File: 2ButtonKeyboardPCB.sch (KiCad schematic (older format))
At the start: 14 parts

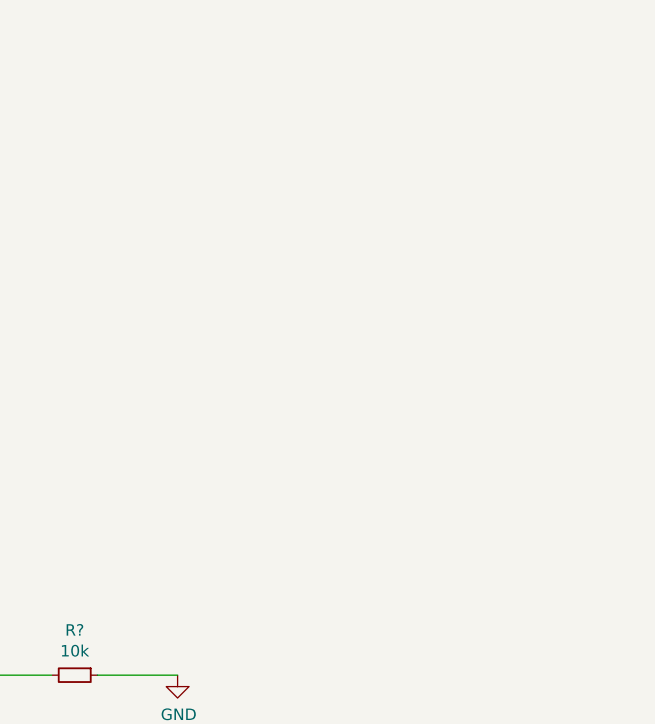
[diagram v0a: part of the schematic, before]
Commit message: Schematic
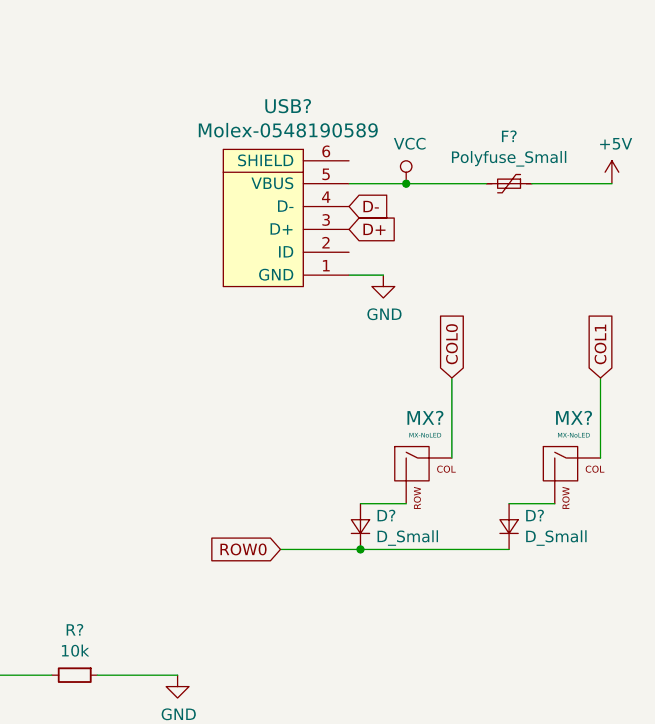
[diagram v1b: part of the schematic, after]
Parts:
- added D? (x2): D_Small, symbol Device:D_Small
- added F?: Polyfuse_Small, symbol Device:Polyfuse_Small
- added MX? (x2): MX-NoLED, symbol MX_Alps_Hybrid:MX-NoLED
- added USB?: Molex-0548190589, symbol random-keyboard-parts:Molex-0548190589
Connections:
- net +5V: now also F?.1
- net D+: now also USB?.3 (D+)
- net D-: now also USB?.4 (D-)
- net GND: now also USB?.1 (GND)
- new net: D?.2 (A), MX?.2 (ROW) (x2)
- new net COL0: MX?.1 (COL)
- new net COL1: MX?.1 (COL)
- new net ROW0: D?.1 (K), D?.1 (K)
- new net VCC: F?.2, USB?.5 (VBUS)
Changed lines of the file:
@@
 Text GLabel 4250 3150 0    50   Input ~ 0
 D-
+$Comp
+L random-keyboard-parts:Molex-0548190589 USB?
+U 1 1 63CE0F7D
+P 8100 2200
+F 0 "USB?" V 8637 2167 60  0000 C CNN
+F 1 "Molex-0548190589" V 8531 2167 60  0000 C CNN
+F 2 "" H 8100 2200 60  0001 C CNN
+F 3 "" H 8100 2200 60  0001 C CNN
+	1    8100 2200
+	0    -1   -1   0
+$EndComp
+$Comp
+L power:VCC #PWR?
+U 1 1 63CE60A6
+P 8650 2000
+F 0 "#PWR?" H 8650 1850 50  0001 C CNN
+F 1 "VCC" H 8667 2173 50  0000 C CNN
+F 2 "" H 8650 2000 50  0001 C CNN
+F 3 "" H 8650 2000 50  0001 C CNN
+	1    8650 2000
+	1    0    0    -1
+$EndComp
+Wire Wire Line
+	8400 2000 8650 2000
+$Comp
+L Device:Polyfuse_Small F?
+U 1 1 63CE9399
+P 9100 2000
+F 0 "F?" V 8895 2000 50  0000 C CNN
+F 1 "Polyfuse_Small" V 8986 2000 50  0000 C CNN
+F 2 "" H 9150 1800 50  0001 L CNN
+F 3 "~" H 9100 2000 50  0001 C CNN
+	1    9100 2000
+	0    1    1    0
+$EndComp
+Wire Wire Line
+	8650 2000 9000 2000
+Connection ~ 8650 2000
+$Comp
+L power:+5V #PWR?
+U 1 1 63CEB500
+P 9550 2000
+F 0 "#PWR?" H 9550 1850 50  0001 C CNN
+F 1 "+5V" H 9565 2173 50  0000 C CNN
+F 2 "" H 9550 2000 50  0001 C CNN
+F 3 "" H 9550 2000 50  0001 C CNN
+	1    9550 2000
+	1    0    0    -1
+$EndComp
+Wire Wire Line
+	9200 2000 9550 2000
+Text GLabel 8400 2200 2    50   Input ~ 0
+D+
+Text GLabel 8400 2100 2    50   Input ~ 0
+D-
+$Comp
+L power:GND #PWR?
+U 1 1 63CED46D
+P 8550 2400
+F 0 "#PWR?" H 8550 2150 50  0001 C CNN
+F 1 "GND" H 8555 2227 50  0000 C CNN
+F 2 "" H 8550 2400 50  0001 C CNN
+F 3 "" H 8550 2400 50  0001 C CNN
+	1    8550 2400
+	1    0    0    -1
+$EndComp
+Wire Wire Line
+	8400 2400 8550 2400
+$Comp
+L MX_Alps_Hybrid:MX-NoLED MX?
+U 1 1 63CEF074
+P 8700 3250
+F 0 "MX?" H 8733 3473 60  0000 C CNN
+F 1 "MX-NoLED" H 8733 3399 20  0000 C CNN
+F 2 "" H 8075 3225 60  0001 C CNN
+F 3 "" H 8075 3225 60  0001 C CNN
+	1    8700 3250
+	1    0    0    -1
+$EndComp
+$Comp
+L Device:D_Small D?
+U 1 1 63CF120D
+P 8450 3500
+F 0 "D?" V 8496 3432 50  0000 R CNN
+F 1 "D_Small" V 8405 3432 50  0000 R CNN
+F 2 "" V 8450 3500 50  0001 C CNN
+F 3 "~" V 8450 3500 50  0001 C CNN
+	1    8450 3500
+	0    -1   -1   0
+$EndComp
+Wire Wire Line
+	8650 3400 8450 3400
+$Comp
+L MX_Alps_Hybrid:MX-NoLED MX?
+U 1 1 63CF6D29
+P 9350 3250
+F 0 "MX?" H 9383 3473 60  0000 C CNN
+F 1 "MX-NoLED" H 9383 3399 20  0000 C CNN
+F 2 "" H 8725 3225 60  0001 C CNN
+F 3 "" H 8725 3225 60  0001 C CNN
+	1    9350 3250
+	1    0    0    -1
+$EndComp
+$Comp
+L Device:D_Small D?
+U 1 1 63CF6D33
+P 9100 3500
+F 0 "D?" V 9146 3432 50  0000 R CNN
+F 1 "D_Small" V 9055 3432 50  0000 R CNN
+F 2 "" V 9100 3500 50  0001 C CNN
+F 3 "~" V 9100 3500 50  0001 C CNN
+	1    9100 3500
+	0    -1   -1   0
+$EndComp
+Wire Wire Line
+	9300 3400 9100 3400
+Wire Wire Line
+	9100 3600 8450 3600
+Connection ~ 8450 3600
+Wire Wire Line
+	8450 3600 8100 3600
+Wire Wire Line
+	8850 3200 8850 2850
+Wire Wire Line
+	9500 3200 9500 2850
+Text GLabel 8850 2850 1    50   Input ~ 0
+COL0
+Text GLabel 9500 2850 1    50   Input ~ 0
+COL1
+Text GLabel 8100 3600 0    50   Input ~ 0
+ROW0
 $EndSCHEMATC
